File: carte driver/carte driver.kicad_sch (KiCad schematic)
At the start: 43 parts, among them J1 UART CP, J10 STEPPER 4, J11 STEPPER 3, J2 Conn_01x03, J3 UART BONUS, J4 Conn_01x02, J6 STEPPER G, J7 STEPPER D, J8 STEPPER 1, J9 STEPPER 2, SW2 SW_DIP_x02, SW3 SW_DIP_x02, SW4 SW_DIP_x02, SW5 SW_DIP_x02, SW6 SW_DIP_x02, SW7 SW_DIP_x02, U1 TMC2209_SILENTSTEPSTICK, U10 XIAO-HALF-HOLE-23P, U2 TMC2209_SILENTSTEPSTICK, U3 TMC2209_SILENTSTEPSTICK, U4 TMC2209_SILENTSTEPSTICK, U5 TMC2209_SILENTSTEPSTICK, U6 TMC2209_SILENTSTEPSTICK

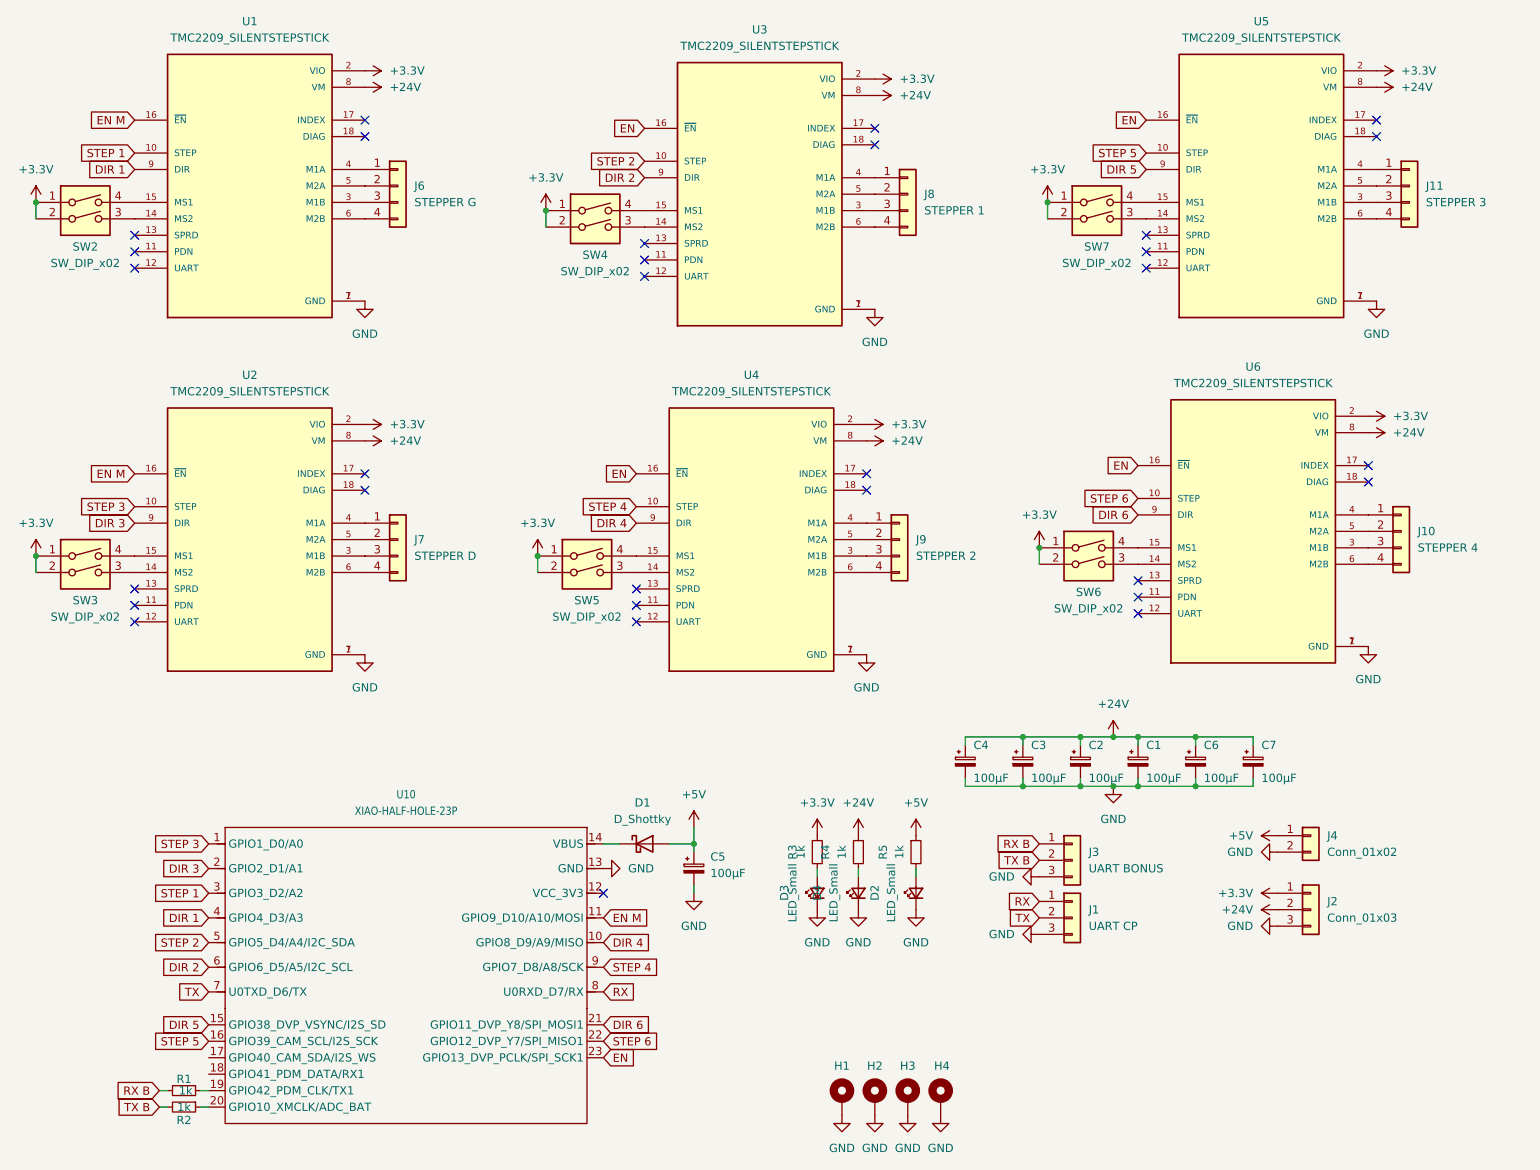
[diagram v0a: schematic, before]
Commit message: apdavph
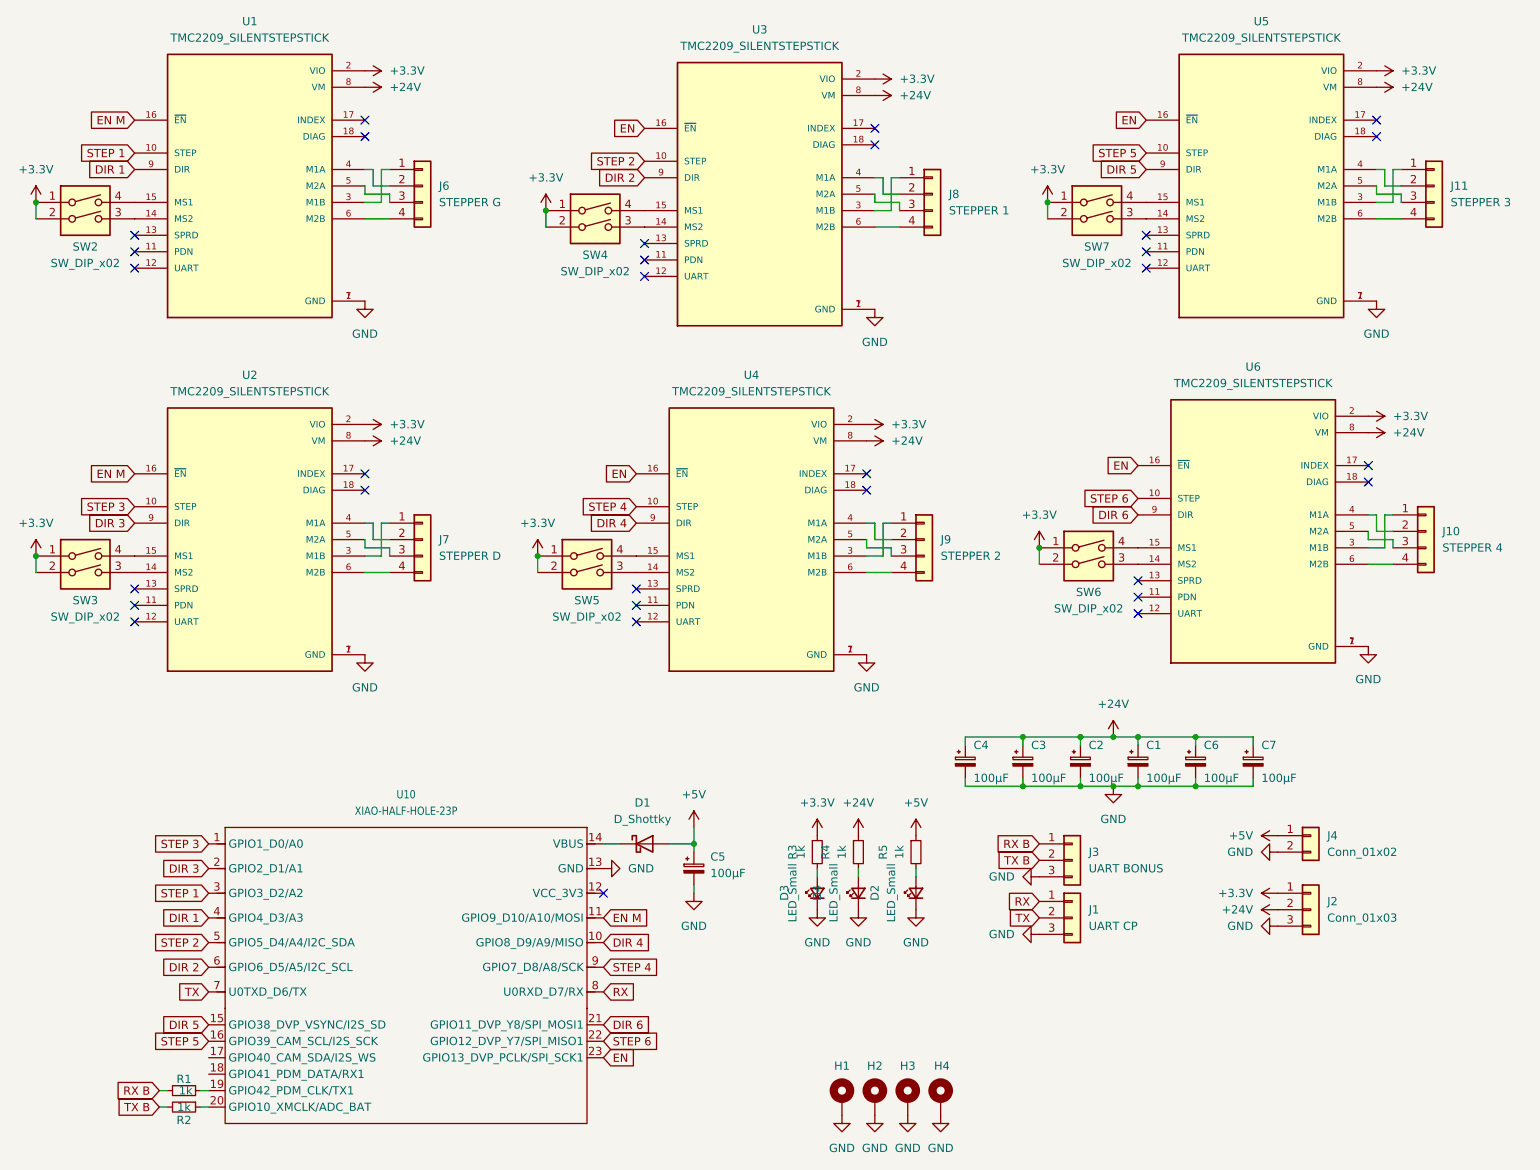
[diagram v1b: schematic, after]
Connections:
- net at U3.3 (M1B): now also J8.1 (Pin_1); no longer J8.3 (Pin_3)
- net at U3.4 (M1A): now also J8.2 (Pin_2); no longer J8.1 (Pin_1)
- net at U3.5 (M2A): now also J8.3 (Pin_3); no longer J8.2 (Pin_2)
- net at U6.3 (M1B): now also J10.1 (Pin_1); no longer J10.3 (Pin_3)
- net at U6.4 (M1A): now also J10.2 (Pin_2); no longer J10.1 (Pin_1)
- net at U6.5 (M2A): now also J10.3 (Pin_3); no longer J10.2 (Pin_2)
- net at J9.1 (Pin_1): now also U4.3 (M1B); no longer U4.4 (M1A)
- net at J9.2 (Pin_2): now also U4.4 (M1A); no longer U4.5 (M2A)
- net at J9.3 (Pin_3): now also U4.5 (M2A); no longer U4.3 (M1B)
- net at J7.1 (Pin_1): now also U2.3 (M1B); no longer U2.4 (M1A)
- net at J7.2 (Pin_2): now also U2.4 (M1A); no longer U2.5 (M2A)
- net at J7.3 (Pin_3): now also U2.5 (M2A); no longer U2.3 (M1B)
- net at U1.3 (M1B): now also J6.1 (Pin_1); no longer J6.3 (Pin_3)
- net at U1.4 (M1A): now also J6.2 (Pin_2); no longer J6.1 (Pin_1)
- net at U1.5 (M2A): now also J6.3 (Pin_3); no longer J6.2 (Pin_2)
- net at J11.1 (Pin_1): now also U5.3 (M1B); no longer U5.4 (M1A)
- net at J11.2 (Pin_2): now also U5.4 (M1A); no longer U5.5 (M2A)
- net at J11.3 (Pin_3): now also U5.5 (M2A); no longer U5.3 (M1B)
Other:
- moved on the sheet: J10, J11, J6, J7, J8, J9
